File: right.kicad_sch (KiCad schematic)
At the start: 66 parts, among them J1 RIGHT, U2 TL072

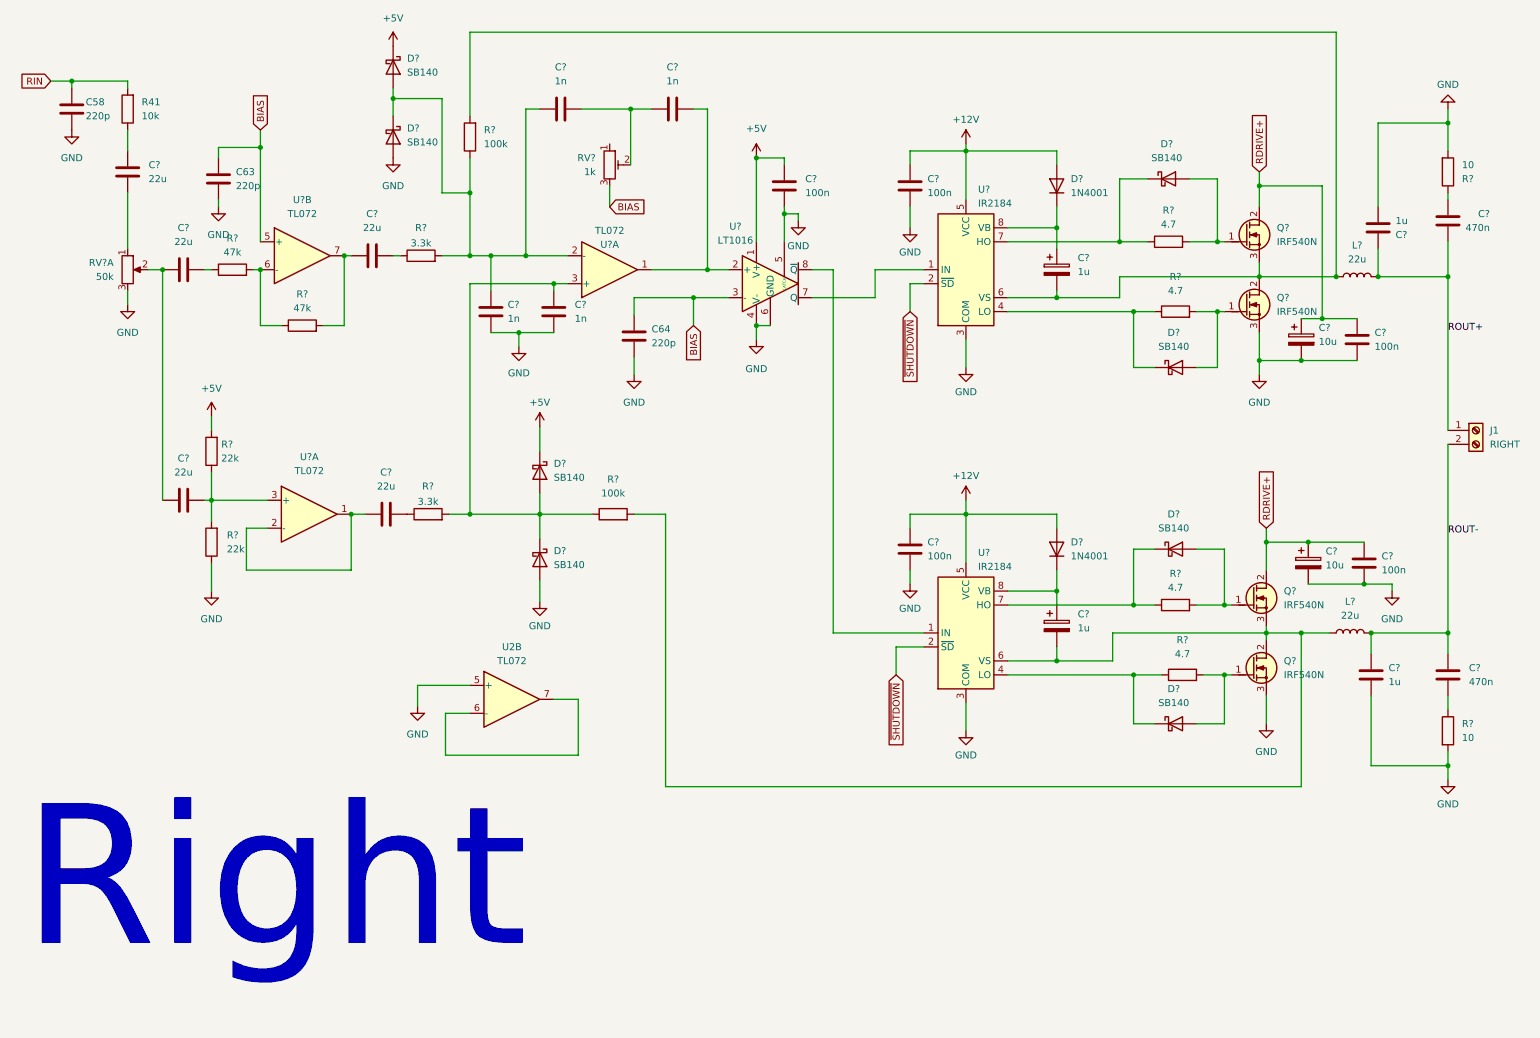
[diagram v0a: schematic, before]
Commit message: WIP
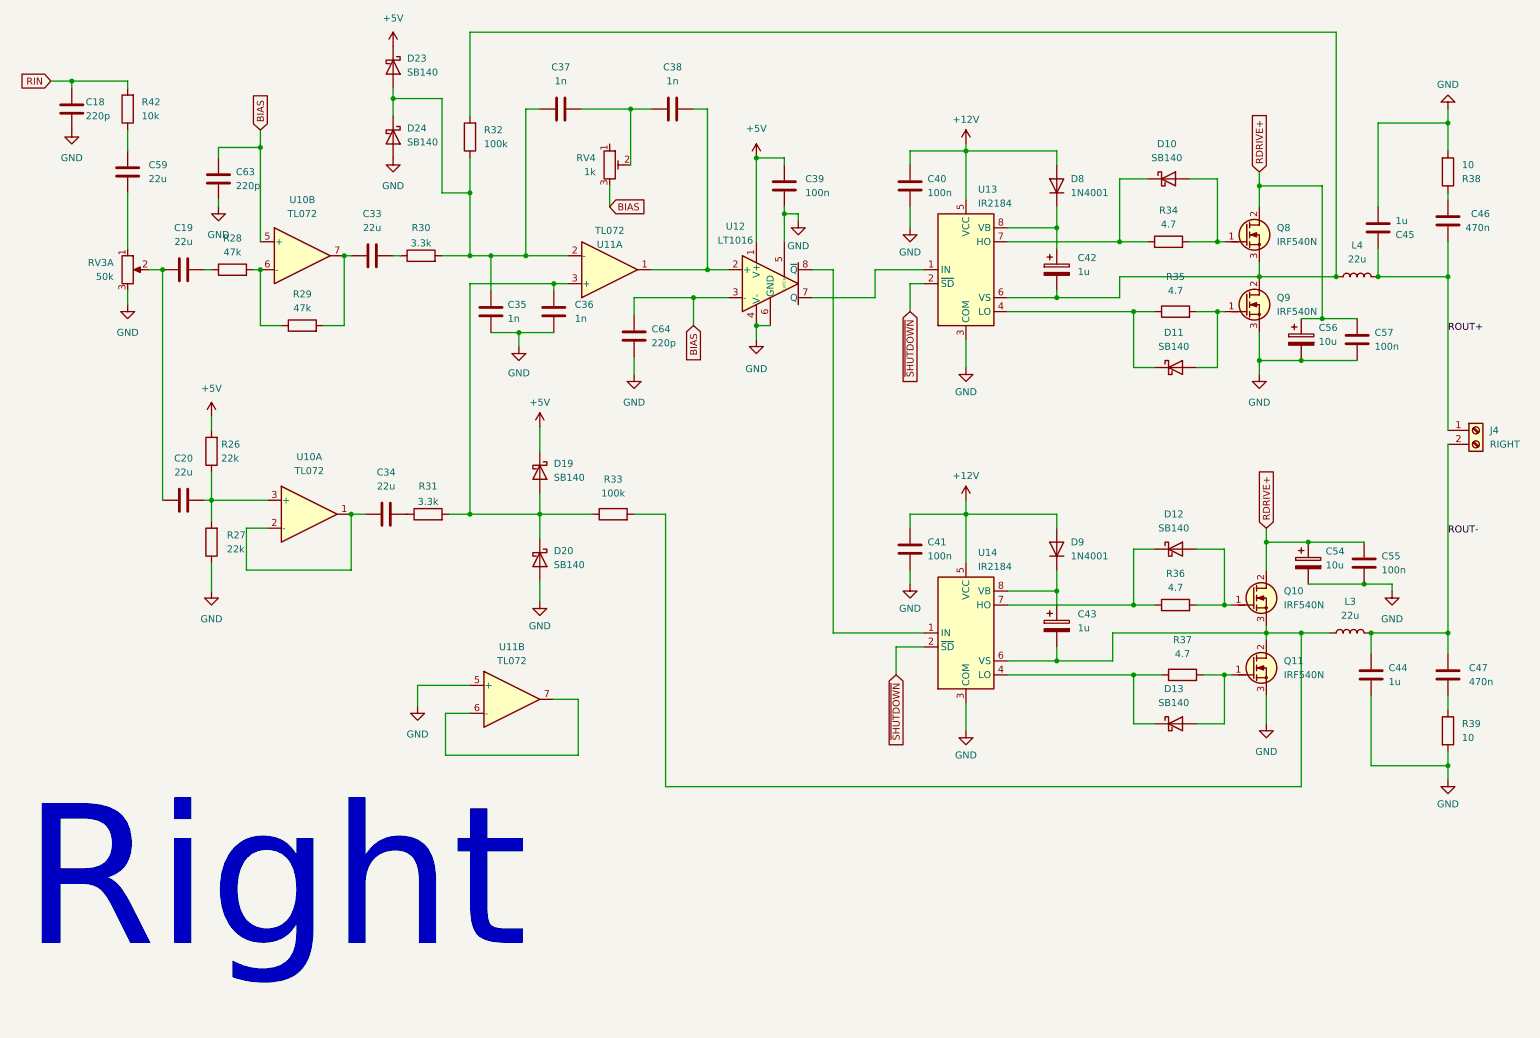
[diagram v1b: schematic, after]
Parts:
- gave numbers to parts that had none: 59
- renumbered C58 to C18, J1 to J4, R41 to R42, U2 to U11

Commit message: Recovered PCB
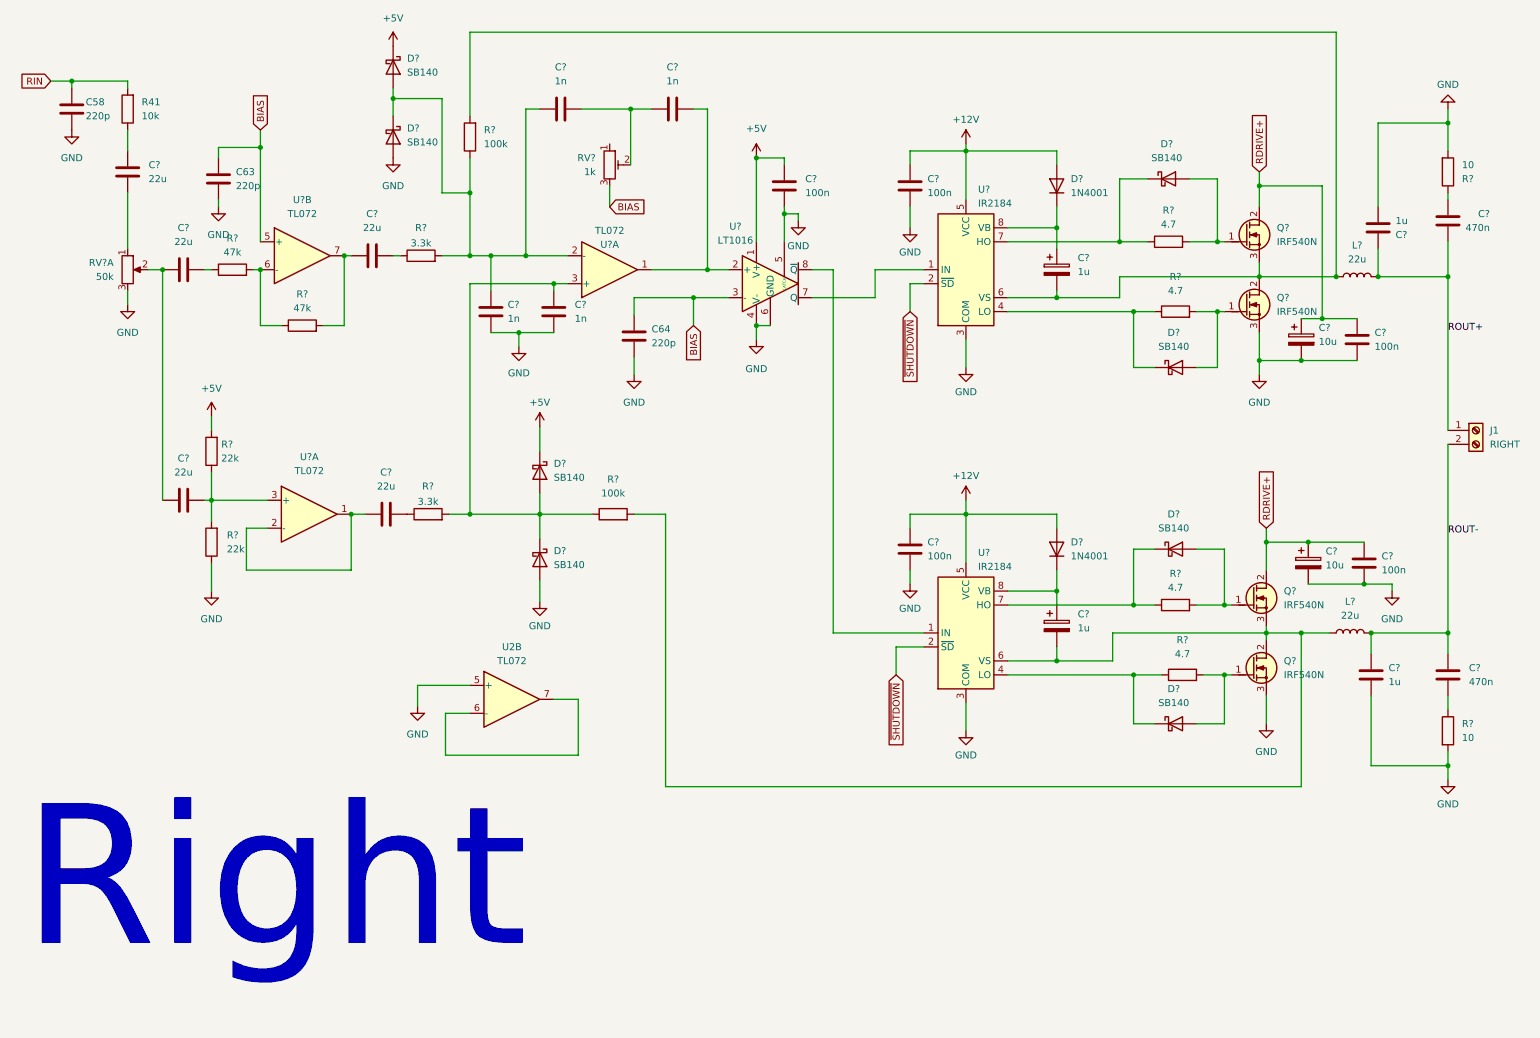
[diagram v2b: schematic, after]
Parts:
- renumbered C18 to C58, C54 to C?, C40 to C?, C43 to C?, C39 to C?, C45 to C?, C37 to C?, C20 to C?, C36 to C?, C19 to C?, C55 to C?, C41 to C?, C59 to C?, C47 to C?, C34 to C?, C33 to C?, C42 to C?, C46 to C?, C35 to C?, C57 to C?, C38 to C?, C44 to C?, C56 to C?, D20 to D?, D13 to D?, D24 to D?, D23 to D?, D8 to D?, D12 to D?, D9 to D?, D11 to D?, D19 to D?, D10 to D?, J4 to J1, L3 to L?, L4 to L?, Q10 to Q?, Q8 to Q?, Q11 to Q?, Q9 to Q?, R42 to R41, R31 to R?, R26 to R?, R30 to R?, R37 to R?, R29 to R?, R28 to R?, R33 to R?, R27 to R?, R36 to R?, R35 to R?, R38 to R?, R32 to R?, R39 to R?, R34 to R?, RV3 to RV?, RV4 to RV?, U11 to U2, U10 to U?, U13 to U?, U11 to U?, U14 to U?, U12 to U?
